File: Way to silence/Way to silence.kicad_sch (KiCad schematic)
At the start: 17 parts, among them J3 5V_Terminal, J4 Battery_Terminal, J5 LEDS Port, SW1 SW_SPDT, SW3 SW_SPST, U1 ESP32-WROOM-32-N16, U6 AMS1117CD-3.3

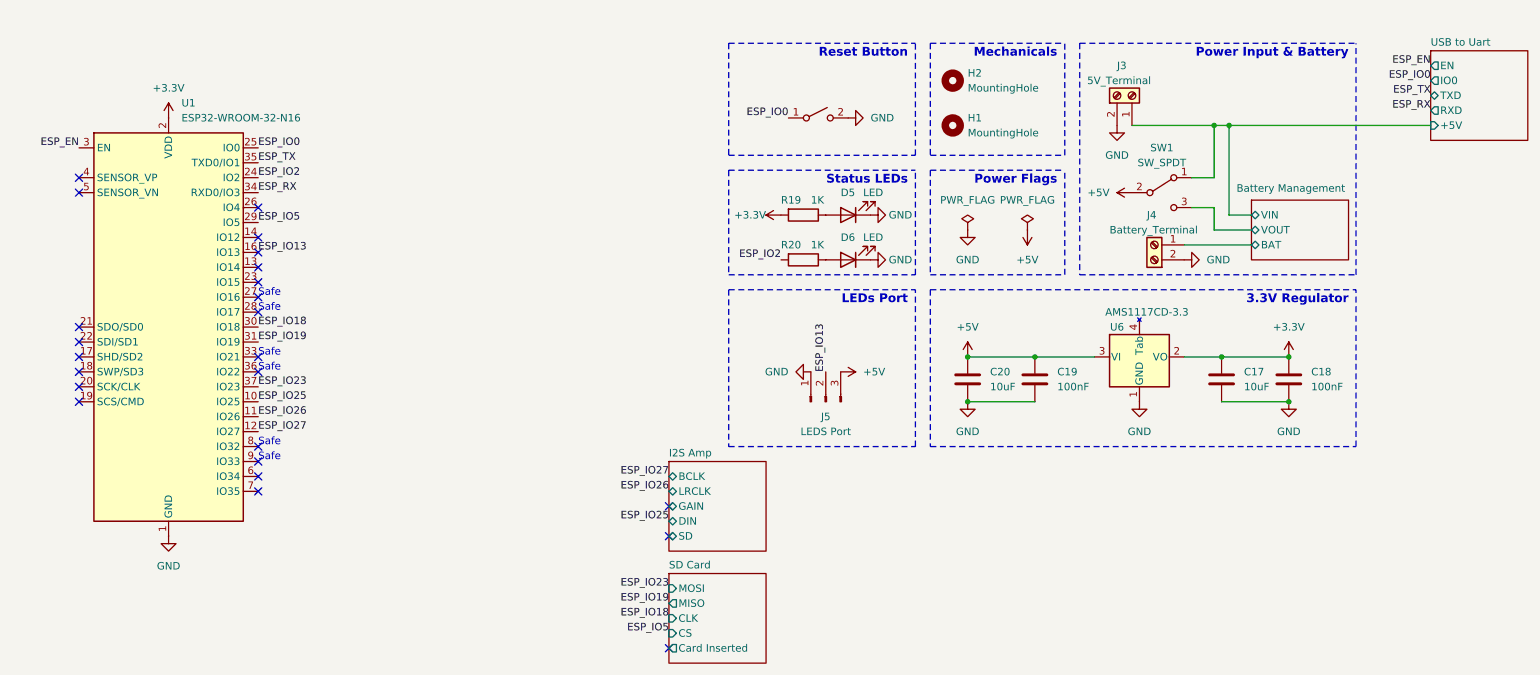
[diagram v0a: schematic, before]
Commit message: [ADD] Root page style
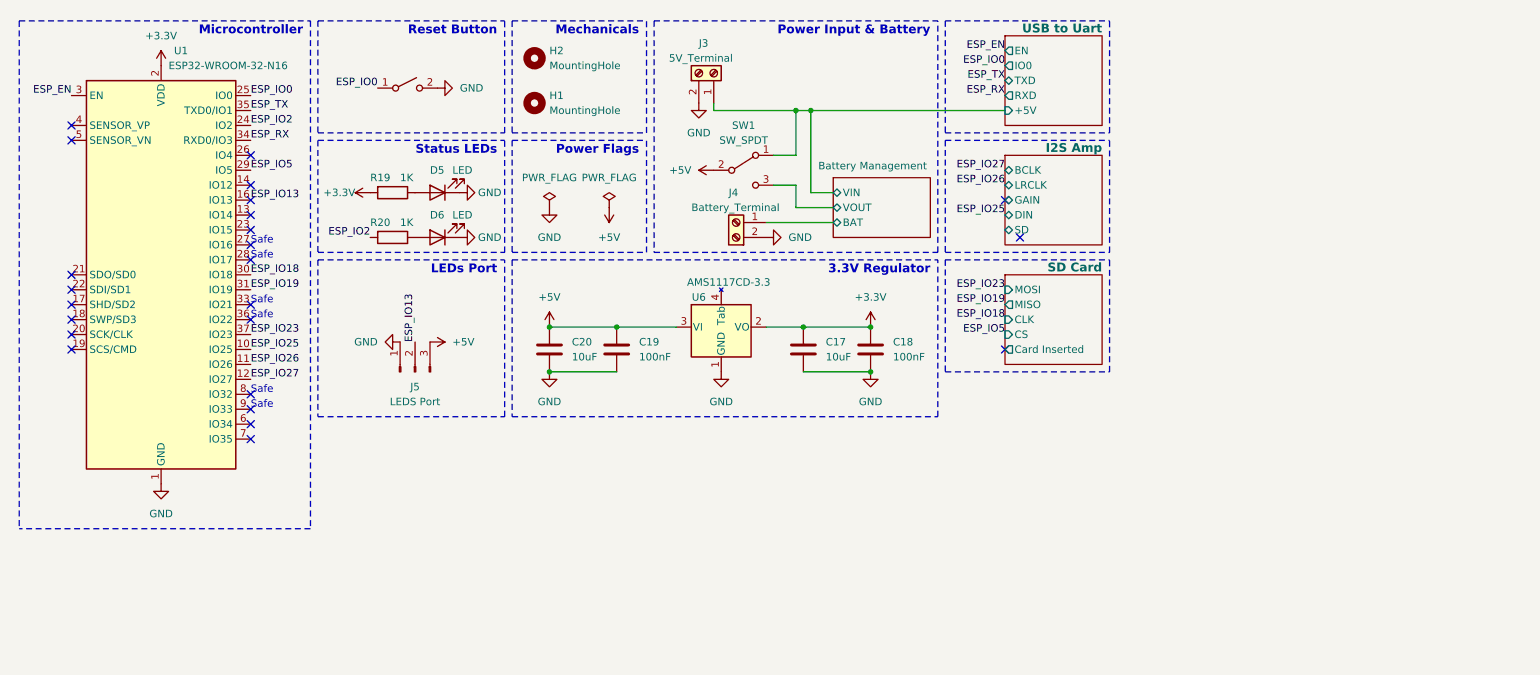
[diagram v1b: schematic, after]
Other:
- note added: "Microcontroller"
- moved on the sheet: C17, C18, C19, C20, D5, D6, H1, H2, J3, J4, J5, R19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

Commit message: [ADD] Shematics files settings
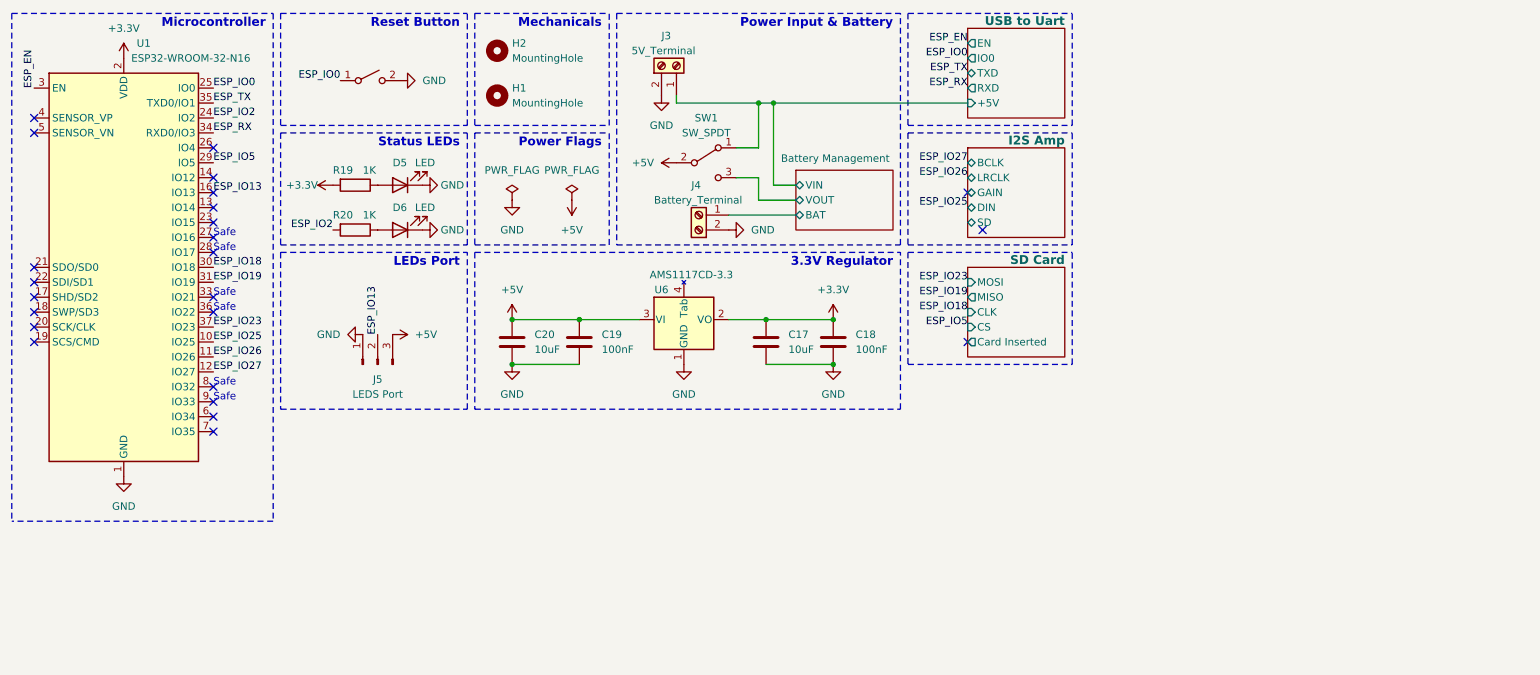
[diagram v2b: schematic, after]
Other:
- title: (none) -> Way To Silence
- moved on the sheet: C17, C18, C19, C20, D5, D6, H1, H2, J3, J4, J5, R19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
